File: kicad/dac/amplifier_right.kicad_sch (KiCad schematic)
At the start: 44 parts, among them Q10 MMBT5551, Q11 BCM53DS, Q12 MMBT5551, Q13 MMBT5551, Q14 MMBT5551, Q15 MMBT5401, Q16 2SC4511, Q17 2SA1725, Q7 BCM53DS, Q8 BCM53DS, Q9 BCM56DS

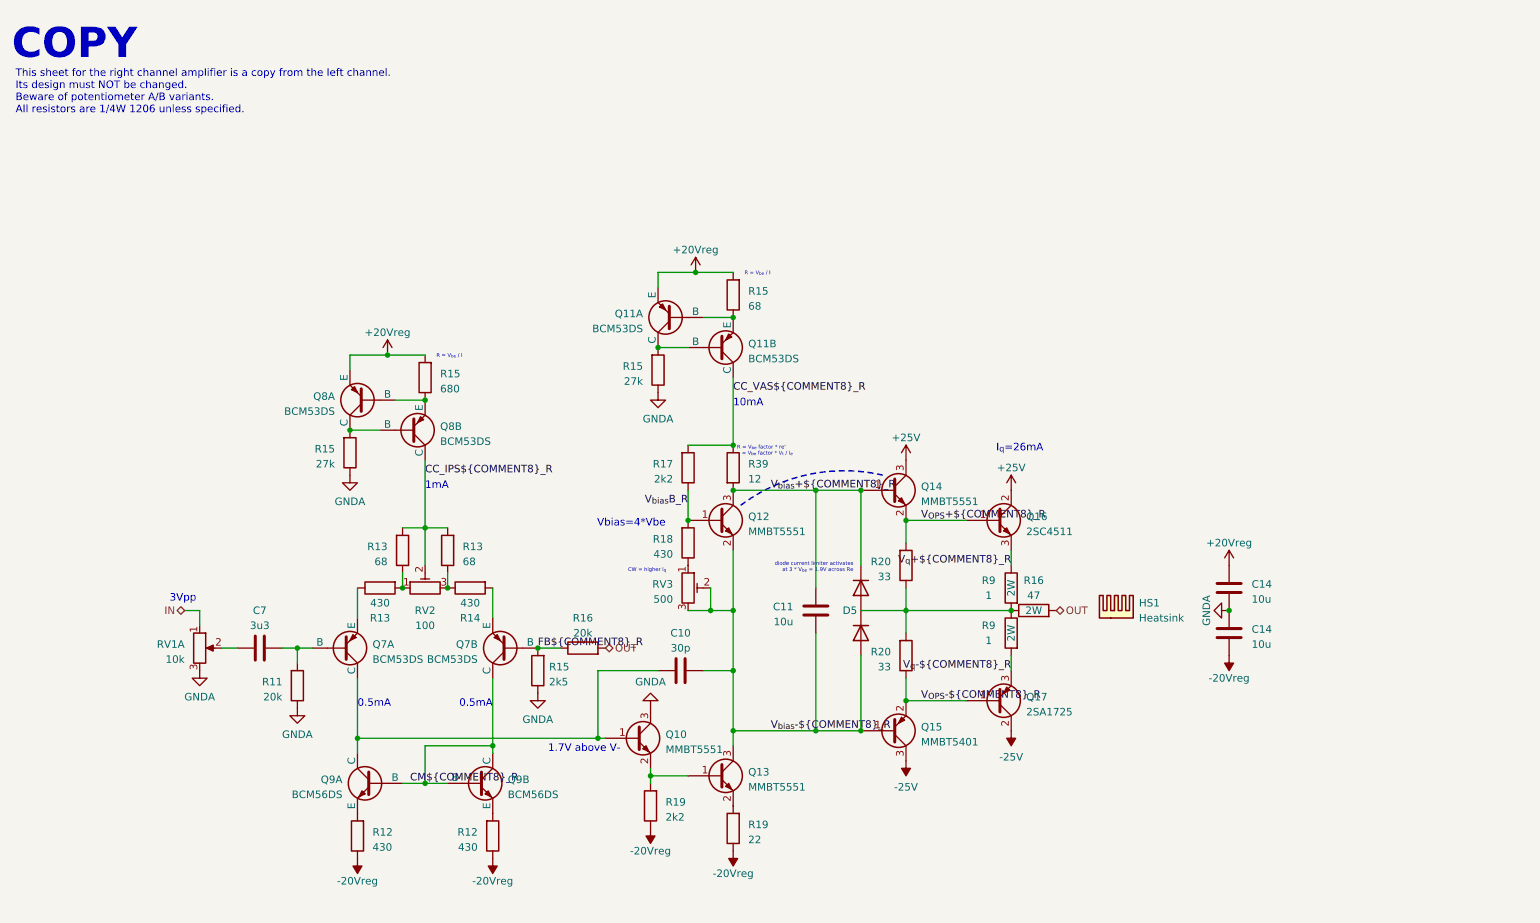
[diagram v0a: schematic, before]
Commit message: commit
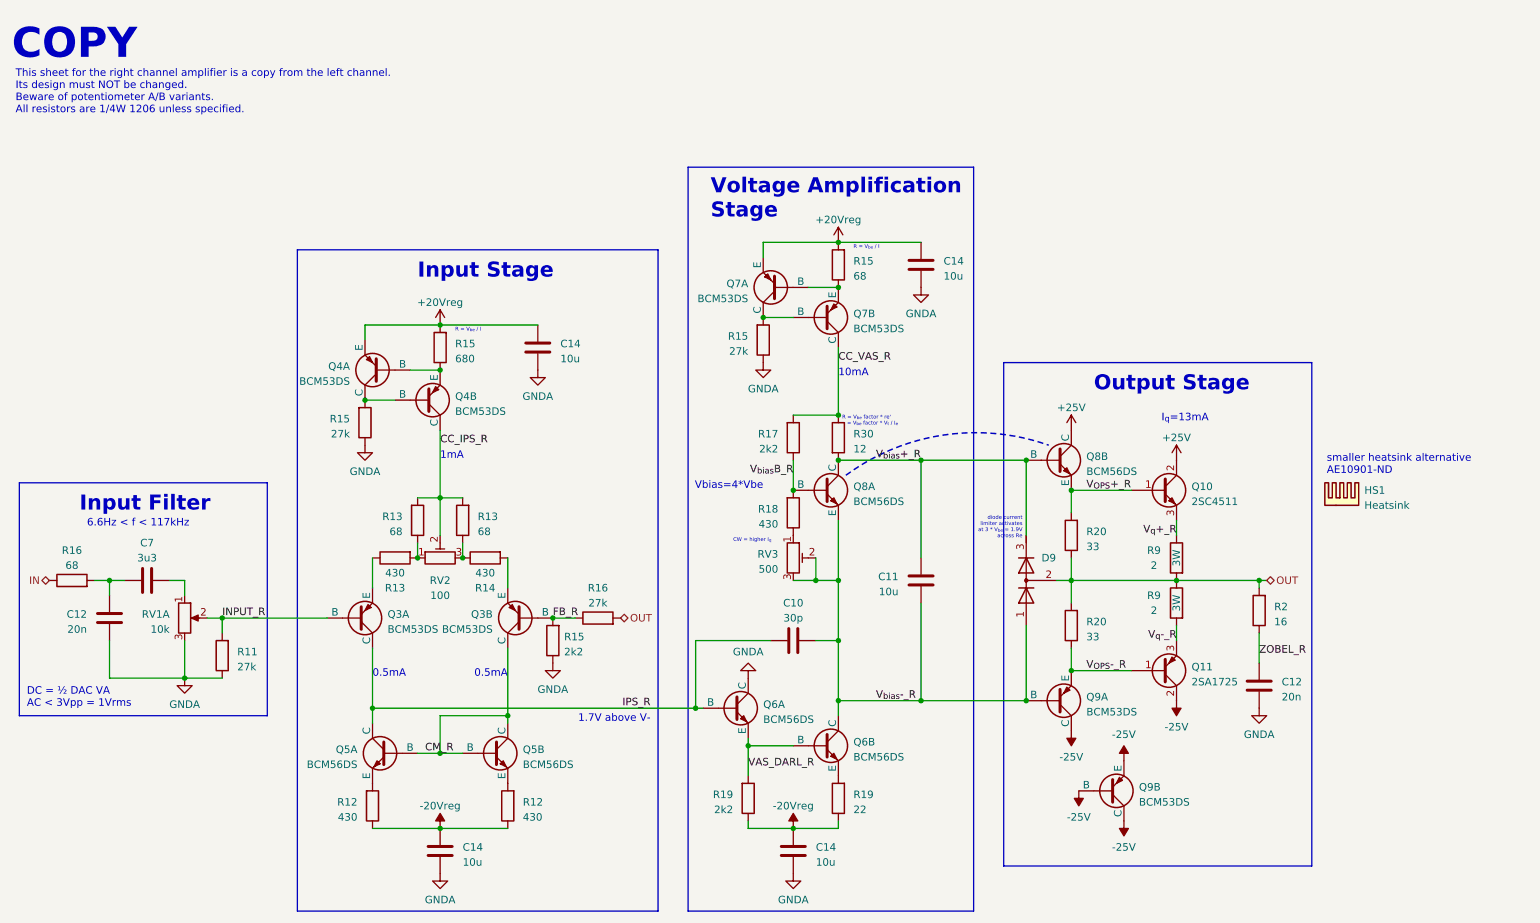
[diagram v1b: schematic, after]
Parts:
- removed C14 (x2): 10u, Capacitor_SMD:C_1206_3216Metric_Pad1.33x1.80mm_HandSolder, symbol Device:C
- removed D5: ~, Package_TO_SOT_SMD:SOT-23-3, symbol library:Dual_Diode_Array
- removed Q10, Q12, Q13, Q14: MMBT5551, Package_TO_SOT_SMD:SOT-23-3, symbol Device:Q_NPN_BEC
- removed Q11, Q8: BCM53DS, Package_SO:SC-74-6_1.5x2.9mm_P0.95mm, symbol library:Dual-PNP
- removed Q15: MMBT5401, Package_TO_SOT_SMD:SOT-23-3, symbol Device:Q_PNP_BEC
- removed Q16: 2SC4511, Package_TO_SOT_THT:TO-220F-3_Vertical, symbol Device:Q_NPN_BCE
- removed Q17: 2SA1725, Package_TO_SOT_THT:TO-220F-3_Vertical, symbol Device:Q_PNP_BCE
- removed Q9: BCM56DS, Package_SO:SC-74-6_1.5x2.9mm_P0.95mm, symbol library:Dual-NPN
- removed R12 (x2), R13: 430, Resistor_SMD:R_1206_3216Metric_Pad1.30x1.75mm_HandSolder, symbol Device:R
- removed R13 (x2), R15: 68, Resistor_SMD:R_1206_3216Metric_Pad1.30x1.75mm_HandSolder, symbol Device:R
- removed R15: 680, Resistor_SMD:R_1206_3216Metric_Pad1.30x1.75mm_HandSolder, symbol Device:R
- removed R15 (x2): 27k, Resistor_SMD:R_1206_3216Metric_Pad1.30x1.75mm_HandSolder, symbol Device:R
- removed R15: 2k5, Resistor_THT:R_Axial_DIN0207_L6.3mm_D2.5mm_P10.16mm_Horizontal, symbol Device:R
- removed R16: 20k, Resistor_THT:R_Axial_DIN0207_L6.3mm_D2.5mm_P10.16mm_Horizontal, symbol Device:R
- removed R16: 47, symbol Device:R
- removed R19: 22, Resistor_SMD:R_1206_3216Metric_Pad1.30x1.75mm_HandSolder, symbol Device:R
- removed R19: 2k2, Resistor_SMD:R_1206_3216Metric_Pad1.30x1.75mm_HandSolder, symbol Device:R
- removed R20 (x2): 33, Resistor_SMD:R_1206_3216Metric_Pad1.30x1.75mm_HandSolder, symbol Device:R
- removed R39: 12, Resistor_SMD:R_1206_3216Metric_Pad1.30x1.75mm_HandSolder, symbol Device:R
- removed R9 (x2): 1, Resistor_THT:R_Axial_DIN0614_L14.3mm_D5.7mm_P20.32mm_Horizontal, symbol Device:R
- added C12 (x2): 20n, Capacitor_SMD:C_1206_3216Metric_Pad1.33x1.80mm_HandSolder, symbol Device:C
- added C14 (x4): 10u, Capacitor_SMD:C_1206_3216Metric_Pad1.33x1.80mm_HandSolder, symbol Device:C
- added D9: ~, Package_TO_SOT_SMD:SOT-23-3, symbol Device:D_Dual_Series_ACK
- added Q10: 2SC4511, Package_TO_SOT_THT:TO-220F-3_Vertical, symbol Device:Q_NPN_BCE
- added Q11: 2SA1725, Package_TO_SOT_THT:TO-220F-3_Vertical, symbol Device:Q_PNP_BCE
- added Q3, Q4, Q9: BCM53DS, Package_SO:SC-74-6_1.5x2.9mm_P0.95mm, symbol library:Dual-PNP
- added Q5, Q6, Q8: BCM56DS, Package_SO:SC-74-6_1.5x2.9mm_P0.95mm, symbol library:Dual-NPN
- added R12 (x2), R13: 430, Resistor_SMD:R_1206_3216Metric_Pad1.30x1.75mm_HandSolder, symbol Device:R
- added R13 (x2), R15, R16: 68, Resistor_SMD:R_1206_3216Metric_Pad1.30x1.75mm_HandSolder, symbol Device:R
- added R15, R19: 2k2, Resistor_SMD:R_1206_3216Metric_Pad1.30x1.75mm_HandSolder, symbol Device:R
- added R15 (x2), R16: 27k, Resistor_SMD:R_1206_3216Metric_Pad1.30x1.75mm_HandSolder, symbol Device:R
- added R15: 680, Resistor_SMD:R_1206_3216Metric_Pad1.30x1.75mm_HandSolder, symbol Device:R
- added R19: 22, Resistor_SMD:R_1206_3216Metric_Pad1.30x1.75mm_HandSolder, symbol Device:R
- added R2: 16, Resistor_SMD:R_1206_3216Metric_Pad1.30x1.75mm_HandSolder, symbol Device:R
- added R20 (x2): 33, Resistor_SMD:R_1206_3216Metric_Pad1.30x1.75mm_HandSolder, symbol Device:R
- added R30: 12, Resistor_SMD:R_1206_3216Metric_Pad1.30x1.75mm_HandSolder, symbol Device:R
- added R9 (x2): 2, Resistor_THT:R_Axial_DIN0614_L14.3mm_D5.7mm_P20.32mm_Horizontal, symbol Device:R
- R11: value 20k -> 27k; footprint Resistor_THT:R_Axial_DIN0207_L6.3mm_D2.5mm_P10.16mm_Horizontal -> Resistor_SMD:R_1206_3216Metric_Pad1.30x1.75mm_HandSolder
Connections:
- net CM${COMMENT8}${COMMENT9} is gone; now on net CC_VAS_R: Q7.3 (C)
- net FB${COMMENT8}${COMMENT9} is gone; now on an unnamed net: Q7.2 (B)
- net +20Vreg: now also Q7.5 (E), C14.1, C14.1, Q4.5 (E), R15.2, R15.2
- net +25V: now also Q10.2 (C), Q8.3 (C)
- net -20Vreg: now also C14.1, C14.1, R12.1, R12.1, R19.1, R19.1
- net -25V: now also Q11.2 (C), Q9.2 (B), Q9.3 (C), Q9.4 (E), Q9.6 (C)
- net GNDA: now also C12.1, C12.1, C14.2, C14.2, C14.2, C14.2, Q6.6 (C), R15.1, R15.1, R15.1
- net IN: now also R16.1; no longer RV1.1
- net OUT: now also D9.2 (common), R16.2, R2.2, R20.1, R20.2, R9.1, R9.2
- net at RV2.1: now also R13.1, R13.2
- net at Q7.6 (C): now also R15.2; no longer C10.1
- net at C7.1: now also C12.2, R16.2; no longer RV1.2
- net at R14.1, RV2.3: now also R13.1
- net at Q7.4 (E): now also Q7.1 (B), R15.1; no longer R14.2
- net CC_IPS${COMMENT8}${COMMENT9} renamed CC_IPS_R
- net CC_IPS_R: now also Q4.3 (C), R13.2, R13.2
- net CC_VAS${COMMENT8}${COMMENT9} renamed CC_VAS_R
- net CC_VAS_R: now also R30.1
- net V_{bias}+${COMMENT8}${COMMENT9} renamed V_{bias}+_R
- net V_{bias}+_R: now also D9.3 (K), Q8.2 (B), Q8.6 (C), R30.2
- net V_{bias}-${COMMENT8}${COMMENT9} renamed V_{bias}-_R
- net V_{bias}-_R: now also D9.1 (A), Q6.3 (C), Q8.5 (E), Q9.1 (B)
- net V_{bias}B${COMMENT9} renamed V_{bias}B_R
- net V_{bias}B_R: now also Q8.1 (B)
- new net: C7.2, RV1.1
- new net: Q4.2 (B), Q4.6 (C), R15.2
- new net: Q4.1 (B), Q4.4 (E), R15.1
- new net: Q5.4 (E), R12.2
- new net: Q6.4 (E), R19.2
- new net: Q3.5 (E), R13.1
- new net: Q5.5 (E), R12.2
- new net: Q3.4 (E), R14.2
- new net CM_R: Q3.3 (C), Q5.1 (B), Q5.2 (B), Q5.3 (C)
- new net FB_R: Q3.2 (B), R15.2, R16.1
- new net INPUT_R: Q3.1 (B), R11.2, RV1.2
- new net IPS_R: C10.1, Q3.6 (C), Q5.6 (C), Q6.1 (B)
- new net VAS_DARL_R: Q6.2 (B), Q6.5 (E), R19.2
- new net V_{OPS}+_R: Q10.1 (B), Q8.4 (E), R20.2
- new net V_{OPS}-_R: Q11.1 (B), Q9.5 (E), R20.1
- new net V_{q}+_R: Q10.3 (E), R9.1
- new net V_{q}-_R: Q11.3 (E), R9.2
- new net ZOBEL_R: C12.2, R2.1
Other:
- note added: "6.6Hz < f < 117kHz"
- note added: "DC = ½ DAC VA AC < 3Vpp = 1Vrms"
- note added: "I_{q}=13mA"
- note added: "Input Filter"
- note added: "Input Stage"
- note added: "Output Stage"
- note added: "Voltage Amplification Stage"
- note added: "smaller heatsink alternative AE10901-ND"
- note removed: "3Vpp"
- note removed: "I_{q}=26mA"
